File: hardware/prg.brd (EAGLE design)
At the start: 50.8 x 23.8 mm, 3 parts, among them IC1 MEGA8-PU

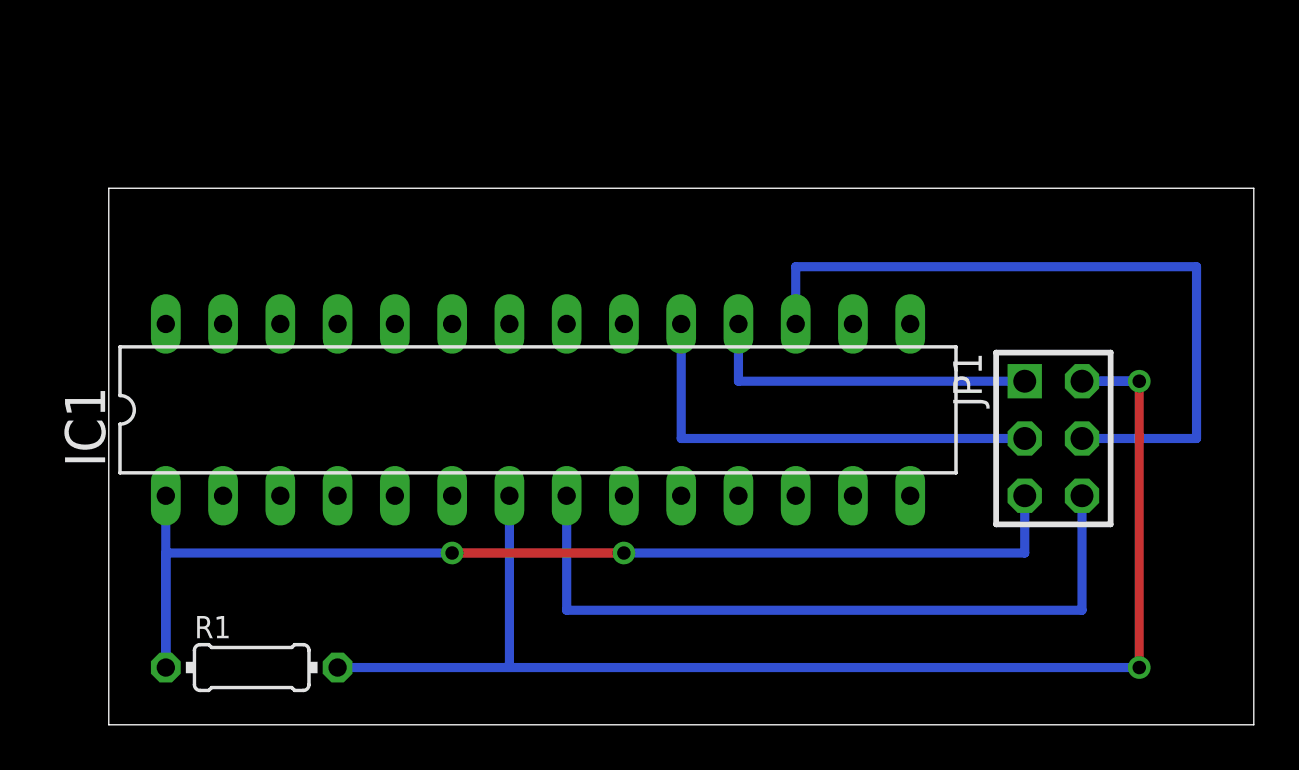
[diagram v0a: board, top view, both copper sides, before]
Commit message: Fixes.
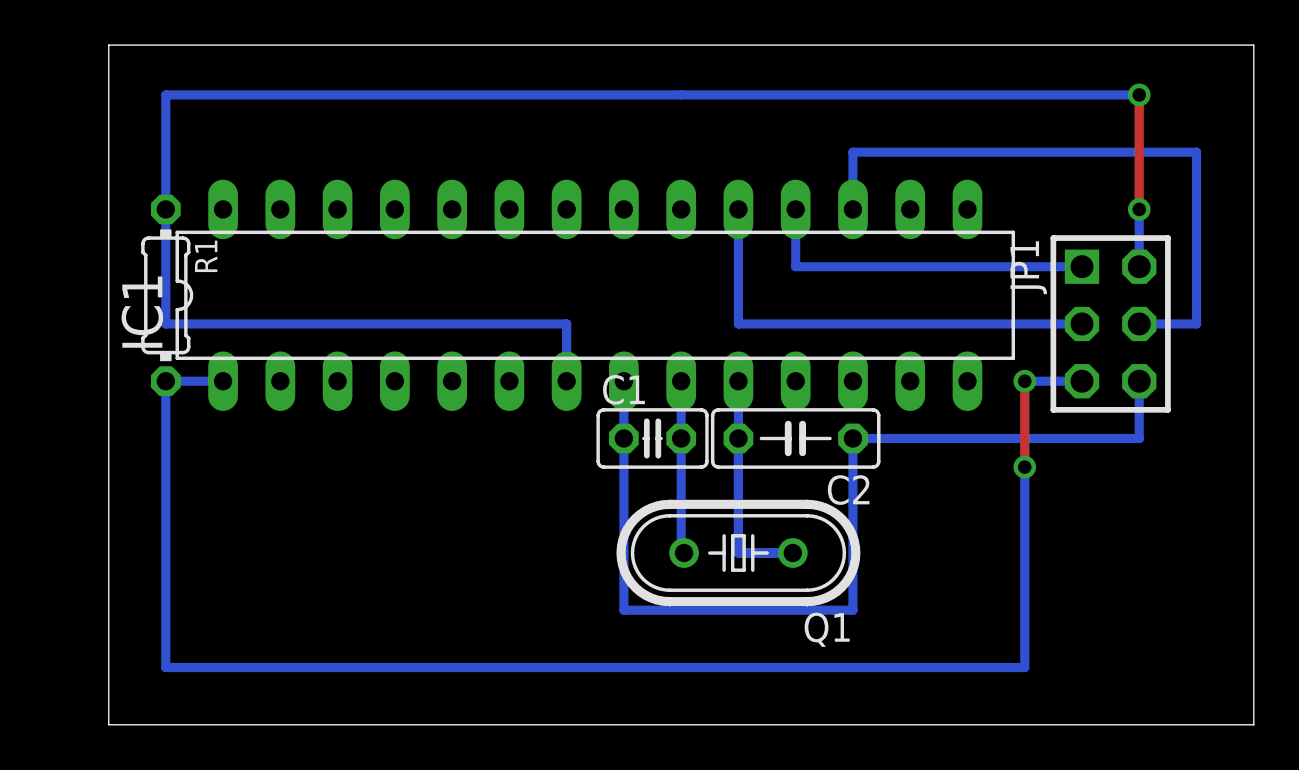
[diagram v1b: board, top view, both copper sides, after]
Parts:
- added C1: 22pF, rcl:C025-025X050
- added C2: 22pF, rcl:C050-025X075
- added Q1: 16MHz, crystal:HC49/S
- moved R1 16.9 mm to (2.54, 19.1), turned to 270 degrees
- moved JP1 5.68 mm to (44.5, 17.8)
- moved IC1 5.68 mm to (21.6, 19.1)
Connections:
- removed net N$6: IC1.1, JP1.5, R1.1
- new net GND: C1.1, C2.1, IC1.8, JP1.6
- new net N$7: IC1.1, JP1.5, R1.2
- new net VCC: IC1.7, JP1.2, R1.1
- net N$4: now also C2.2, IC1.10, Q1.1; no longer IC1.8, JP1.6
- net N$5: now also C1.2, IC1.9, Q1.2; no longer IC1.7, JP1.2, R1.2
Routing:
- net VCC: track 0.00 -> 81.3 mm, vias 0 -> 2
- net N$7: track 0.00 -> 68.6 mm, vias 0 -> 2
- net N$6: track 53.3 -> 0.00 mm, vias 2 -> 0
- net N$5: track 61.0 -> 7.75 mm, vias 2 -> 0
- net GND: track 0.00 -> 43.2 mm
- net N$4: track 33.0 -> 17.5 mm
- net N$2: track 33.0 -> 27.9 mm
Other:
- board size 50.8 x 23.8 mm -> 50.8 x 30.1 mm
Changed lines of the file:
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@@
 <board>
 <plain>
-<wire x1="50.8" y1="0" x2="50.8" y2="23.8" width="0" layer="20"/>
-<wire x1="50.8" y1="23.8" x2="0.01" y2="23.8" width="0" layer="20"/>
-<wire x1="0.01" y1="23.8" x2="0.01" y2="0" width="0" layer="20"/>
+<wire x1="50.8" y1="0" x2="50.8" y2="30.15" width="0" layer="20"/>
+<wire x1="50.8" y1="30.15" x2="0.01" y2="30.15" width="0" layer="20"/>
+<wire x1="0.01" y1="30.15" x2="0.01" y2="0" width="0" layer="20"/>
 <wire x1="0.01" y1="0" x2="50.8" y2="0" width="0" layer="20"/>
-<dimension x1="0.01" y1="0" x2="50.8" y2="0" x3="25.405" y3="-2.54" textsize="1.778" layer="20"/>
-<dimension x1="0.01" y1="0" x2="0" y2="24.13" x3="-2.535" y3="12.063946875" textsize="1.778" layer="20"/>
+<dimension x1="0.01" y1="0" x2="50.8" y2="0" x3="25.405" y3="-2.53999375" textsize="1.778" layer="20"/>
+<dimension x1="0.01" y1="0" x2="0" y2="30.48" x3="-2.53500625" y3="15.239165625" textsize="1.778" layer="20"/>
 </plain>
 <attributes>
@@
 </autorouter>
 <elements>
-<element name="IC1" library="avr-6" package="DIL28-3" value="MEGA8-PU" x="19.05" y="13.97"/>
-<element name="JP1" library="avr-6" package="AVR-ISP-6" value="AVR-ISP-6" x="41.91" y="12.7" rot="R270"/>
-<element name="R1" library="rcl" package="0204/7" value="10k" x="6.35" y="2.54"/>
+<element name="IC1" library="avr-6" package="DIL28-3" value="MEGA8-PU" x="21.59" y="19.05"/>
+<element name="JP1" library="avr-6" package="AVR-ISP-6" value="AVR-ISP-6" x="44.45" y="17.78" rot="R270"/>
+<element name="R1" library="rcl" package="0204/7" value="10k" x="2.54" y="19.05" rot="R270"/>
+<element name="Q1" library="crystal" package="HC49/S" value="16MHz" x="27.94" y="7.62" rot="R180">
+<attribute name="OC_NEWARK" value="unknown" x="27.94" y="7.62" size="1.778" layer="27" rot="R180" display="off"/>
+<attribute name="MPN" value="" x="27.94" y="7.62" size="1.778" layer="27" rot="R180" display="off"/>
+<attribute name="MF" value="" x="27.94" y="7.62" size="1.778" layer="27" rot="R180" display="off"/>
+<attribute name="OC_FARNELL" value="1667008" x="27.94" y="7.62" size="1.778" layer="27" rot="R180" display="off"/>
+</element>
+<element name="C1" library="rcl" package="C025-025X050" value="22pF" x="24.13" y="12.7"/>
+<element name="C2" library="rcl" package="C050-025X075" value="22pF" x="30.48" y="12.7" rot="R180"/>
 </elements>
 <signals>
@@
 <contactref element="JP1" pad="3"/>
 <contactref element="IC1" pad="19"/>
-<wire x1="25.4" y1="17.78" x2="25.4" y2="12.7" width="0.4064" layer="16"/>
-<wire x1="25.4" y1="12.7" x2="40.64" y2="12.7" width="0.4064" layer="16"/>
+<wire x1="27.94" y1="22.86" x2="27.94" y2="17.78" width="0.4064" layer="16"/>
+<wire x1="27.94" y1="17.78" x2="43.18" y2="17.78" width="0.4064" layer="16"/>
 </signal>
 <signal name="N$2">
 <contactref element="JP1" pad="4"/>
 <contactref element="IC1" pad="17"/>
-<wire x1="43.18" y1="12.7" x2="48.26" y2="12.7" width="0.4064" layer="16"/>
-<wire x1="48.26" y1="12.7" x2="48.26" y2="20.32" width="0.4064" layer="16"/>
-<wire x1="48.26" y1="20.32" x2="30.48" y2="20.32" width="0.4064" layer="16"/>
-<wire x1="30.48" y1="20.32" x2="30.48" y2="17.78" width="0.4064" layer="16"/>
+<wire x1="45.72" y1="17.78" x2="48.26" y2="17.78" width="0.4064" layer="16"/>
+<wire x1="48.26" y1="17.78" x2="48.26" y2="25.4" width="0.4064" layer="16"/>
+<wire x1="48.26" y1="25.4" x2="33.02" y2="25.4" width="0.4064" layer="16"/>
+<wire x1="33.02" y1="25.4" x2="33.02" y2="22.86" width="0.4064" layer="16"/>
 </signal>
 <signal name="N$3">
 <contactref element="JP1" pad="1"/>
 <contactref element="IC1" pad="18"/>
-<wire x1="27.94" y1="17.78" x2="27.94" y2="15.24" width="0.4064" layer="16"/>
-<wire x1="27.94" y1="15.24" x2="40.64" y2="15.24" width="0.4064" layer="16"/>
+<wire x1="30.48" y1="22.86" x2="30.48" y2="20.32" width="0.4064" layer="16"/>
+<wire x1="30.48" y1="20.32" x2="43.18" y2="20.32" width="0.4064" layer="16"/>
+</signal>
+<signal name="GND">
+<contactref element="IC1" pad="8"/>
+<contactref element="C2" pad="1"/>
+<contactref element="C1" pad="1"/>
+<contactref element="JP1" pad="6"/>
+<wire x1="45.72" y1="12.7" x2="45.72" y2="15.24" width="0.4064" layer="16"/>
+<wire x1="45.72" y1="12.7" x2="33.02" y2="12.7" width="0.4064" layer="16"/>
+<wire x1="22.86" y1="12.7" x2="22.86" y2="15.24" width="0.4064" layer="16"/>
+<wire x1="22.86" y1="12.7" x2="22.86" y2="5.08" width="0.4064" layer="16"/>
+<wire x1="22.86" y1="5.08" x2="33.02" y2="5.08" width="0.4064" layer="16"/>
+<wire x1="33.02" y1="5.08" x2="33.02" y2="12.7" width="0.4064" layer="16"/>
+</signal>
+<signal name="VCC">
+<contactref element="IC1" pad="7"/>
+<contactref element="JP1" pad="2"/>
+<contactref element="R1" pad="1"/>
+<wire x1="45.72" y1="20.32" x2="45.72" y2="22.86" width="0.4064" layer="16"/>
+<via x="45.72" y="22.86" extent="1-16" drill="0.6" shape="square"/>
+<wire x1="45.72" y1="22.86" x2="45.72" y2="27.94" width="0.4064" layer="1"/>
+<via x="45.72" y="27.94" extent="1-16" drill="0.6" shape="square"/>
+<wire x1="45.72" y1="27.94" x2="25.4" y2="27.94" width="0.4064" layer="16"/>
+<wire x1="25.4" y1="27.94" x2="2.54" y2="27.94" width="0.4064" layer="16"/>
+<wire x1="2.54" y1="27.94" x2="2.54" y2="22.86" width="0.4064" layer="16"/>
+<wire x1="20.32" y1="15.24" x2="20.32" y2="17.78" width="0.4064" layer="16"/>
+<wire x1="20.32" y1="17.78" x2="2.54" y2="17.78" width="0.4064" layer="16"/>
+<wire x1="2.54" y1="17.78" x2="2.54" y2="22.86" width="0.4064" layer="16"/>
 </signal>
 <signal name="N$4">
-<contactref element="JP1" pad="6"/>
-<contactref element="IC1" pad="8"/>
-<wire x1="20.32" y1="10.16" x2="20.32" y2="5.08" width="0.4064" layer="16"/>
-<wire x1="20.32" y1="5.08" x2="43.18" y2="5.08" width="0.4064" layer="16"/>
-<wire x1="43.18" y1="5.08" x2="43.18" y2="10.16" width="0.4064" layer="16"/>
+<contactref element="IC1" pad="10"/>
+<contactref element="Q1" pad="1"/>
+<contactref element="C2" pad="2"/>
+<wire x1="30.353" y1="7.62" x2="27.94" y2="7.62" width="0.4064" layer="16"/>
+<wire x1="27.94" y1="7.62" x2="27.94" y2="12.7" width="0.4064" layer="16"/>
+<wire x1="27.94" y1="12.7" x2="27.94" y2="15.24" width="0.4064" layer="16"/>
+<wire x1="30.353" y1="7.62" x2="27.94" y2="7.62" width="0.4064" layer="16"/>
+<wire x1="27.94" y1="7.62" x2="27.94" y2="12.7" width="0.4064" layer="16"/>
 </signal>
 <signal name="N$5">
-<contactref element="JP1" pad="2"/>
-<contactref element="IC1" pad="7"/>
+<contactref element="IC1" pad="9"/>
+<contactref element="Q1" pad="2"/>
+<contactref element="C1" pad="2"/>
+<wire x1="25.527" y1="7.62" x2="25.4" y2="7.62" width="0.4064" layer="16"/>
+<wire x1="25.4" y1="7.62" x2="25.4" y2="12.7" width="0.4064" layer="16"/>
+<wire x1="25.4" y1="15.24" x2="25.4" y2="12.7" width="0.4064" layer="16"/>
+</signal>
+<signal name="N$7">
+<contactref element="IC1" pad="1"/>
 <contactref element="R1" pad="2"/>
-<wire x1="43.18" y1="15.24" x2="45.72" y2="15.24" width="0.4064" layer="16"/>
-<wire x1="45.72" y1="2.54" x2="17.78" y2="2.54" width="0.4064" layer="16"/>
-<wire x1="17.78" y1="2.54" x2="10.16" y2="2.54" width="0.4064" layer="16"/>
-<wire x1="17.78" y1="10.16" x2="17.78" y2="2.54" width="0.4064" layer="16"/>
-<via x="45.72" y="2.54" extent="1-16" drill="0.6" shape="square"/>
-<wire x1="45.72" y1="2.54" x2="45.72" y2="15.24" width="0.4064" layer="1"/>
-<via x="45.72" y="15.24" extent="1-16" drill="0.6" shape="square"/>
-<wire x1="45.72" y1="15.24" x2="43.18" y2="15.24" width="0.4064" layer="16"/>
-</signal>
-<signal name="N$6">
-<contactref element="IC1" pad="1"/>
-<contactref element="R1" pad="1"/>
 <contactref element="JP1" pad="5"/>
-<wire x1="2.54" y1="10.16" x2="2.54" y2="2.54" width="0.4064" layer="16"/>
-<wire x1="2.54" y1="2.54" x2="2.54" y2="7.62" width="0.4064" layer="16"/>
-<wire x1="2.54" y1="7.62" x2="15.24" y2="7.62" width="0.4064" layer="16"/>
-<via x="15.24" y="7.62" extent="1-16" drill="0.6" shape="square"/>
-<wire x1="15.24" y1="7.62" x2="22.86" y2="7.62" width="0.4064" layer="1"/>
-<via x="22.86" y="7.62" extent="1-16" drill="0.6" shape="square"/>
-<wire x1="22.86" y1="7.62" x2="40.64" y2="7.62" width="0.4064" layer="16"/>
-<wire x1="40.64" y1="7.62" x2="40.64" y2="10.16" width="0.4064" layer="16"/>
+<wire x1="2.54" y1="15.24" x2="5.08" y2="15.24" width="0.4064" layer="16"/>
+<wire x1="40.64" y1="2.54" x2="2.54" y2="2.54" width="0.4064" layer="16"/>
+<wire x1="2.54" y1="2.54" x2="2.54" y2="15.24" width="0.4064" layer="16"/>
+<wire x1="43.18" y1="15.24" x2="40.64" y2="15.24" width="0.4064" layer="16"/>
+<via x="40.64" y="15.24" extent="1-16" drill="0.6" shape="square"/>
+<wire x1="40.64" y1="15.24" x2="40.64" y2="11.43" width="0.4064" layer="1"/>
+<via x="40.64" y="11.43" extent="1-16" drill="0.6" shape="square"/>
+<wire x1="40.64" y1="11.43" x2="40.64" y2="2.54" width="0.4064" layer="16"/>
 </signal>
 </signals>
